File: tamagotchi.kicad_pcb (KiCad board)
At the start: 2 copper layers, 68.7 x 75.9 mm, 11 parts, among them SW1 SW_Push, SW2 SW_Push, SW3 SW_Push, U1 XIAO-ESP32-C3-SMD, U2 HS96L03W2C03

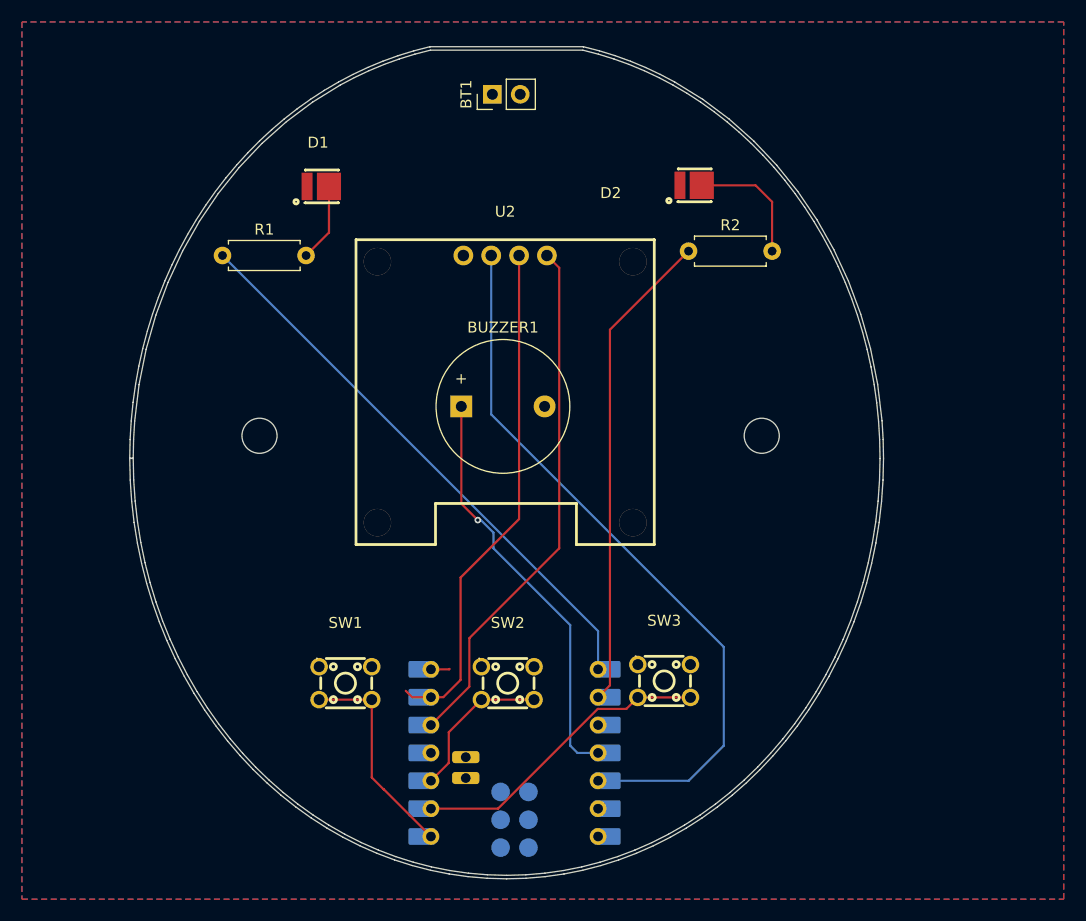
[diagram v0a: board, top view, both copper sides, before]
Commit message: Add files via upload
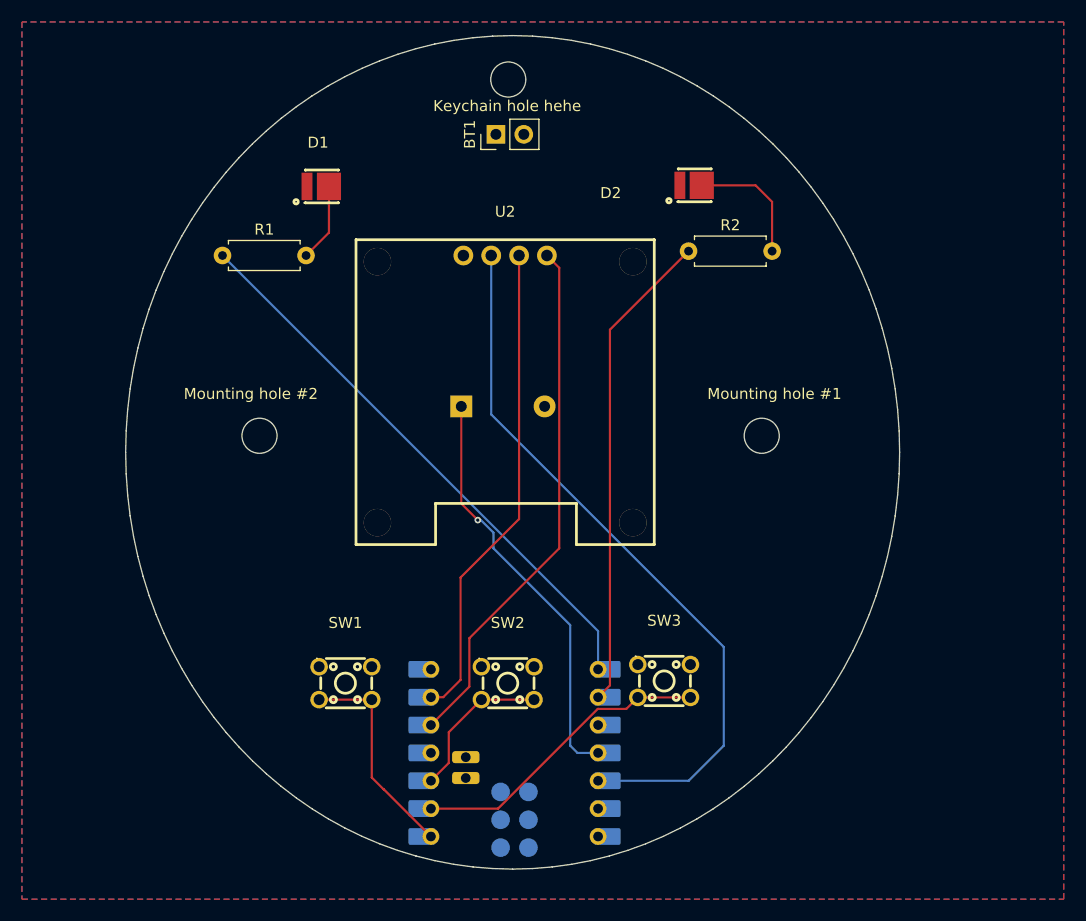
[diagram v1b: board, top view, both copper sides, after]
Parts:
- BUZZER1: moved to B.Cu
- moved BT1 3.66 mm to (148.2, 65.2)
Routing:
- net Net-(U1-GPIO7_D5_SCL): track 46.8 -> 44.3 mm
- net unconnected-(U1-GPIO21_D6_TX-Pad7): track 1.72 -> 0.00 mm
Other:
- board size 68.7 x 75.9 mm -> 70.6 x 76 mm
- board text added: "Keychain hole hehe"
- board text added: "Mounting hole #1"
- board text added: "Mounting hole #2"
